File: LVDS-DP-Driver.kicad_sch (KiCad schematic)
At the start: 122 parts, among them J1 47272-0001, J2 Conn_02x15_Odd_Even, J3 Conn_01x06_Male, J4 Conn_01x03_Male, J5 Conn_01x04_Male, J6 Conn_01x03_Male, Q1 Si4816BDY, Q10 2N7002, Q2 Si4816BDY, Q3 Si4816BDY, Q4 MMBT3904, Q5 MMBT3904, Q6 2N7002, Q7 AO3401A, Q8 2N7002, Q9 2N7002, SW1 SW_DIP_x04, U1 CS5211, U2 LTC3853, U3 AT24C64

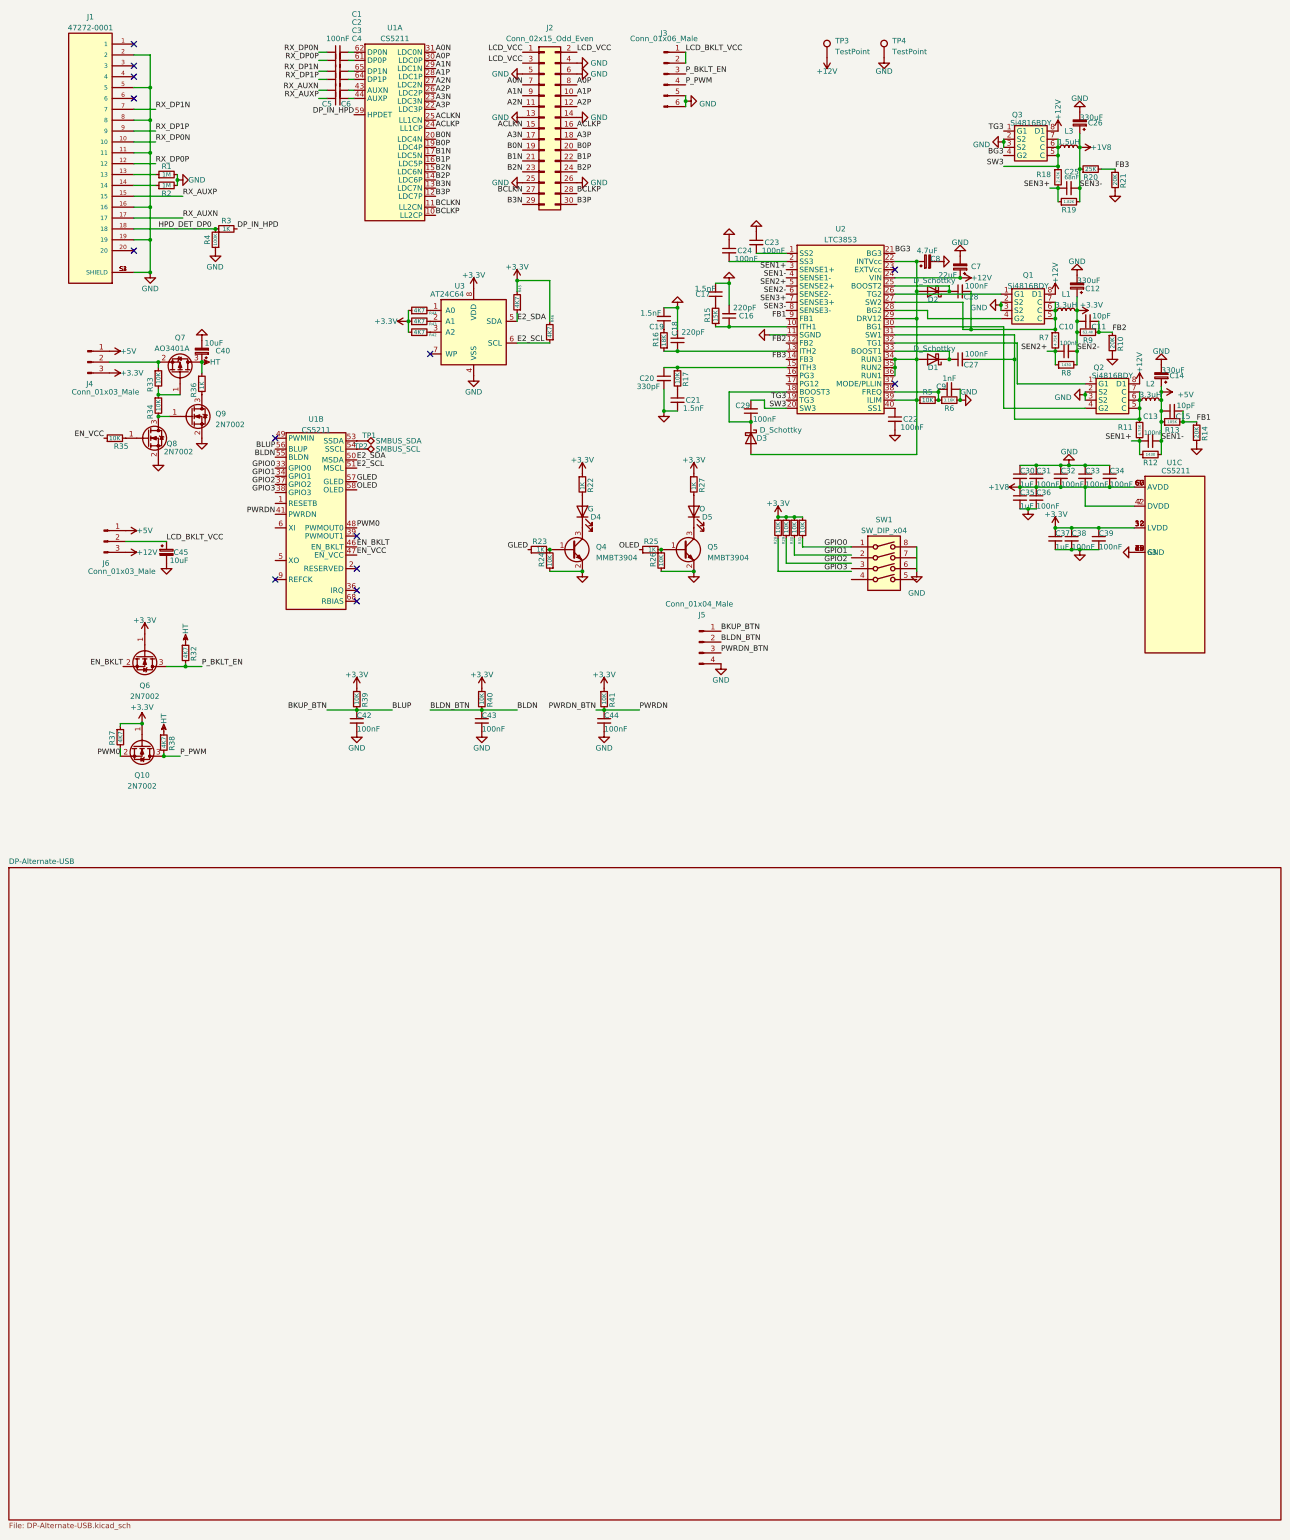
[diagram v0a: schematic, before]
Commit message: cleanup and reconstruct
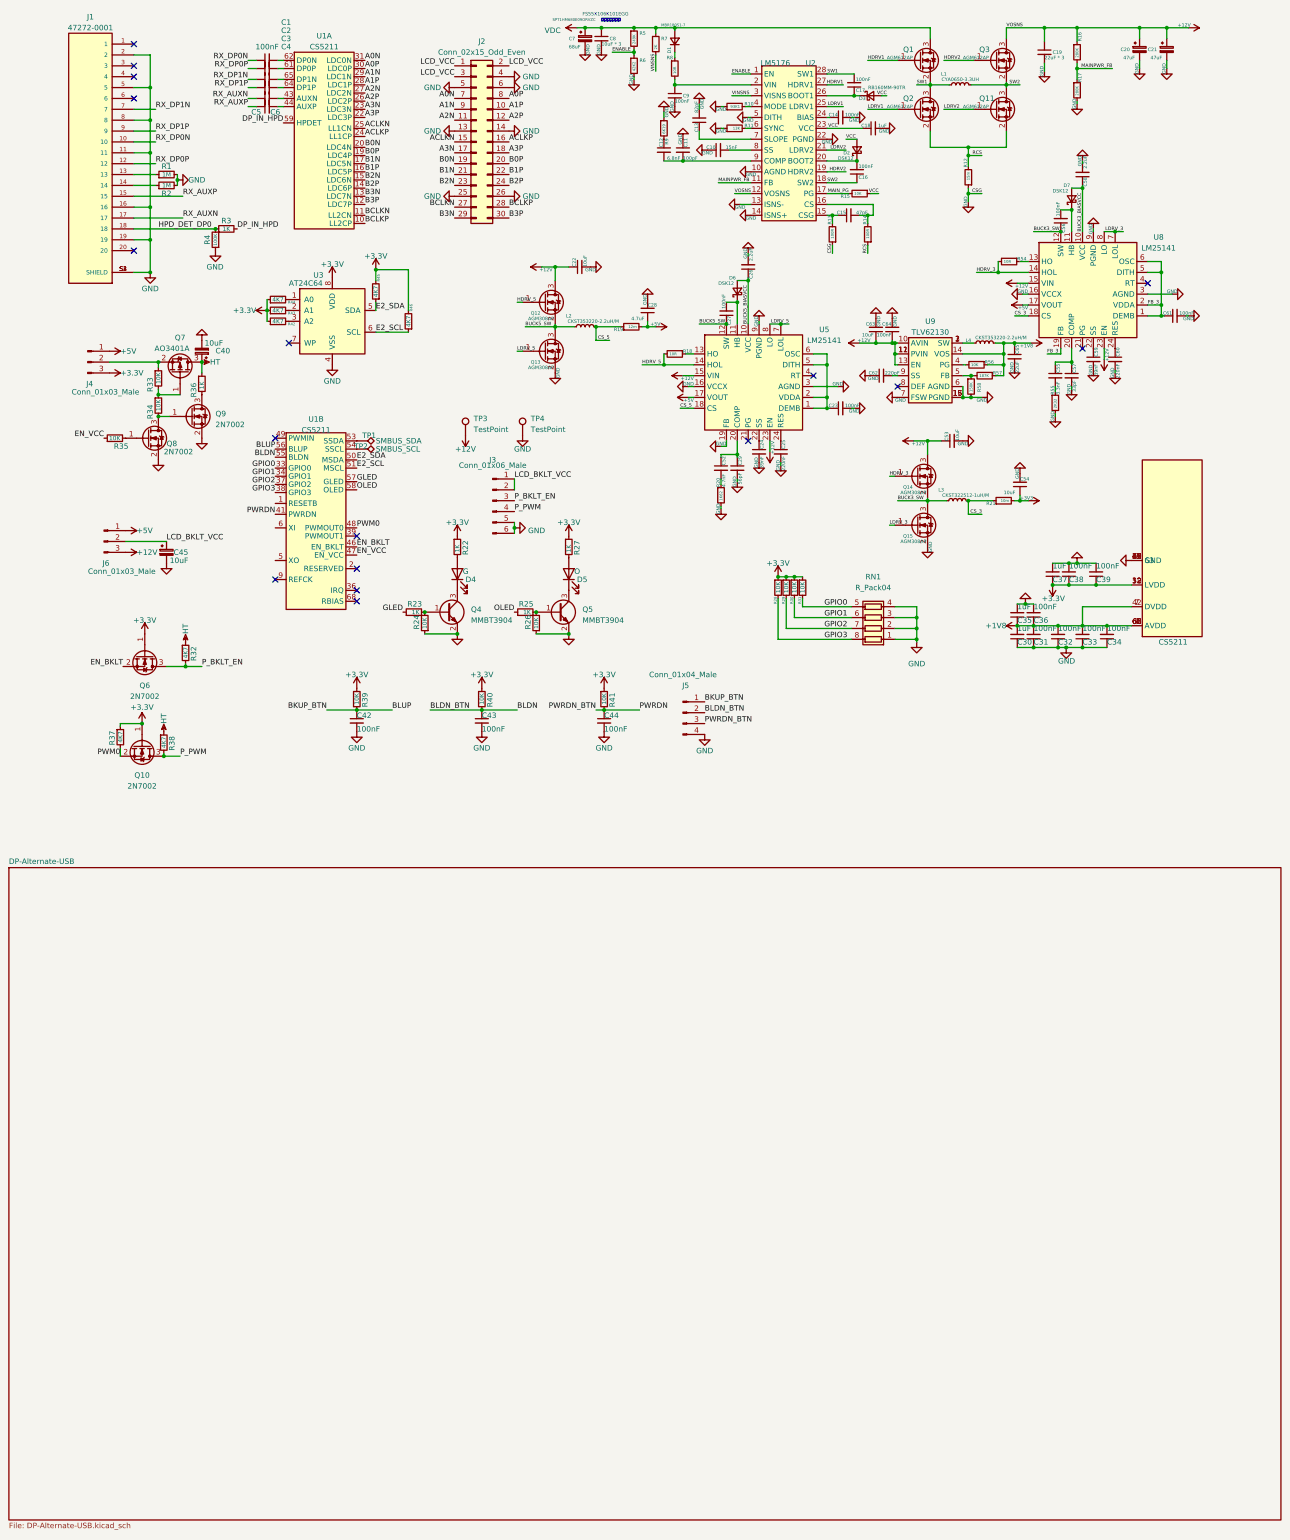
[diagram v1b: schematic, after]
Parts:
- removed C12, C14, C26: 330uF, Capacitor_Tantalum_SMD:CP_EIA-7343-31_Kemet-D, symbol Device:C_Polarized_Small
- removed C20: 330pF, Capacitor_SMD:C_0603_1608Metric, symbol Device:C_Small
- removed C21: 1.5nF, Capacitor_SMD:C_0603_1608Metric, symbol Device:C_Small
- removed C8: 4.7uF, Capacitor_Tantalum_SMD:CP_EIA-3528-21_Kemet-B, symbol Device:C_Polarized_Small
- removed D1, D2, D3: D_Schottky, Diode_SMD:D_SOD-523, symbol Device:D_Schottky
- removed Q1, Q2, Q3: Si4816BDY, Package_SO:SO-8_3.9x4.9mm_P1.27mm, symbol Symbols:Si4816BDY
- removed SW1: SW_DIP_x04, Button_Switch_THT:SW_DIP_SPSTx04_Slide_6.7x11.72mm_W7.62mm_P2.54mm_LowProfile, symbol Switch:SW_DIP_x04
- removed U2: LTC3853, Package_DFN_QFN:QFN-40-1EP_6x6mm_P0.5mm_EP4.6x4.6mm, symbol Symbols:LTC3853
- added C12: 6.8nF, Capacitor_SMD:C_0603_1608Metric, symbol Device:C_Small
- added C14, C56, C61, C64: 100nF, Capacitor_SMD:C_0603_1608Metric, symbol Device:C_Small
- added C20, C21: 47uF, Capacitor_SMD:C_1210_3225Metric, symbol Device:C_Polarized_Small
- added C26, C58: 2.2uF, Capacitor_SMD:C_0603_1608Metric, symbol Device:C_Small
- added C52: 4.7nF, Capacitor_SMD:C_0603_1608Metric, symbol Device:C_Small
- added C53, C54, C63: 10uF, Capacitor_SMD:C_0603_1608Metric, symbol Device:C_Small
- added C55: 3.3nF, Capacitor_SMD:C_0603_1608Metric, symbol Device:C_Small
- added C57: 33pF, Capacitor_SMD:C_0603_1608Metric, symbol Device:C_Small
- added C59: 39nF, Capacitor_SMD:C_0603_1608Metric, symbol Device:C_Small
- added C60: 220nF, Capacitor_SMD:C_0603_1608Metric, symbol Device:C_Small
- added C62: 220pF, Capacitor_SMD:C_0603_1608Metric, symbol Device:C_Small
- added C65: 22uF, Capacitor_SMD:C_0603_1608Metric, symbol Device:C_Small
- added C8: 10uF * 3, Capacitor_SMD:C_2220_5650Metric, symbol Device:C_Small
- added D1: MBR180S1-7, symbol Device:D_Small
- added D2, D6, D7: DSK12, Diode_SMD:D_SOD-123F, symbol Device:D_Schottky_Small
- added D3: RB160MM-90TR, Diode_SMD:D_SOD-123F, symbol Device:D_Schottky_Small
- added L4: CKST353220-2.2uH/M, symbol Device:L_Small
- added Q1, Q11, Q2, Q3: AGM612AP, symbol Device:Q_NMOS_GSD
- added Q12, Q13, Q14, Q15: AGM308AP, symbol Device:Q_NMOS_GSD
- added R54: 10R, symbol Device:R_Small
- added R55: 2K32, symbol Device:R_Small
- added R56: 10K, symbol Device:R_Small
- added R57: 187K, symbol Device:R_Small
- added R58: 150K, symbol Device:R_Small
- added RN1: R_Pack04, symbol Device:R_Pack04
- added U2: LM5176, symbol Symbols:LM5176
- added U5, U8: LM25141, symbol Symbols:LM25141
- added U9: TLV62130, symbol Symbols:TLV62130
- C10: value 100nF -> 15nF
- C11: value 10pF -> 100pF
- C13: value 100nF -> 82pF
- C15: value 10pF -> 47pF
- C16: value 220pF -> 100nF
- C17: value 1.5nF -> 100nF
- C18: value 220pF -> 1uF
- C19: value 1.5nF -> 22uF * 3; footprint Capacitor_SMD:C_0603_1608Metric -> Capacitor_SMD:C_0805_2012Metric
- C22: value 100nF -> 10uF
- C24: value 100nF -> 39nF
- C25: value 68nF -> 220nF
- C28: value 100nF -> 4.7uF
- C29: value 100nF -> 56pF
- C7: value 22uF -> 68uF; footprint Capacitor_Tantalum_SMD:CP_EIA-3528-21_Kemet-B -> Capacitor_THT:CP_Radial_D6.3mm_P2.50mm
- C9: value 1nF -> 100nF
- J1: footprint MOLEX_47272-0001 -> Footprints:MOLEX_47272-0001
- L1: value 3.3uH -> CYA0650-3.3UH; footprint Inductor_SMD:L_7.3x7.3_H4.5 -> (none)
- L2: value 3.3uH -> CKST353220-2.2uH/M; footprint Inductor_SMD:L_7.3x7.3_H4.5 -> (none)
- L3: value 1.5uH -> CKST322512-1uH/M; footprint Inductor_SMD:L_1210_3225Metric -> (none)
- R10: value 20K -> 93K1; footprint Resistor_SMD:R_0603_1608Metric -> (none)
- R11: value 4.75K -> 13K; footprint Resistor_SMD:R_0603_1608Metric -> (none)
- R12: value 1430 -> 15m; footprint Resistor_SMD:R_1206_3216Metric -> (none)
- R13: value 105K -> 100R; footprint Resistor_SMD:R_0603_1608Metric -> (none)
- R14: value 20K -> 100R; footprint Resistor_SMD:R_0603_1608Metric -> (none)
- R15: value 15K -> 10K; footprint Resistor_SMD:R_0603_1608Metric -> (none)
- R16: value 18K -> 280K; footprint Resistor_SMD:R_0603_1608Metric -> (none)
- R17: value 10K -> 280K; footprint Resistor_SMD:R_0603_1608Metric -> (none)
- R18: value 2.43K -> 10R; footprint Resistor_SMD:R_0603_1608Metric -> (none)
- R19: value 1.82K -> 12m; footprint Resistor_SMD:R_0603_1608Metric -> (none)
- R20: value 25K -> 1K62; footprint Resistor_SMD:R_0603_1608Metric -> (none)
- R21: value 20K -> 10m; footprint Resistor_SMD:R_0603_1608Metric -> (none)
- R5: value 10K -> 249K; footprint Resistor_SMD:R_0603_1608Metric -> (none)
- R6: value 3.16K -> 42K2; footprint Resistor_SMD:R_0603_1608Metric -> (none)
- R7: value 4.75K -> 2K; footprint Resistor_SMD:R_0603_1608Metric -> (none)
- R8: value 1430 -> 10R; footprint Resistor_SMD:R_1206_3216Metric -> (none)
- R9: value 63.4K -> 6K19; footprint Resistor_SMD:R_0603_1608Metric -> (none)
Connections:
- net +12V: now also C19.1, C22.1, R16.1, C20.1, C21.1, C53.1, C63.1, C64.1, Q12.3 (D), Q14.3 (D), Q3.3 (D), U2.12 (VOSNS), U5.15 (VIN), U5.23 (EN), U8.15 (VIN), U8.23 (EN), U9.10 (AVIN), U9.11 (PVIN), U9.12 (PVIN), U9.13 (EN); no longer C7.1
- net +1V8: now also C65.1, L4.2, R56.1, R57.1, U9.14 (VOS); no longer C25.2, L3.2, R19.2, R20.1
- net +3.3V: no longer C10.2, C11.1, L1.2, R8.2, R9.1
- net +5V: now also C28.1, R19.2, U5.17 (VOUT), U8.17 (VOUT); no longer C13.2, C15.1, L2.2, R12.2, R13.1
- net GND: now also C10.1, C11.1, C13.2, C23.2, C24.2, C25.2, C28.2, C29.2, R10.1, R11.1, R12.1, R13.1, R17.2, R20.2, R9.1, C14.2, C20.2, C21.2, C26.2, C53.2, C54.2, C57.2, C58.2, C59.2, C60.2, C61.2, C62.1, C63.2, C64.2, C65.2, C8.2, Q13.2 (S), Q15.2 (S), R55.2, R58.2, RN1.1 (R1.1), RN1.2 (R2.1), RN1.3 (R3.1), RN1.4 (R4.1), U2.10 (AGND), U2.13 (ISNS-), U2.14 (ISNS+), U2.22 (PGND), U2.5 (DITH), U5.16 (VCCX), U5.19 (FB), U5.3 (AGND), U5.9 (PGND), U8.16 (VCCX), U8.3 (AGND), U8.9 (PGND), U9.15 (PGND), U9.16 (PGND), U9.17 (PGND), U9.6 (AGND), U9.7 (FSW); no longer C16.2, C17.2, C23.1, C24.1, R10.2, R14.2, R21.2
- net GPIO0: now also RN1.5 (R4.2)
- net GPIO1: now also RN1.6 (R3.2)
- net GPIO2: now also RN1.7 (R2.2)
- net GPIO3: now also RN1.8 (R1.2)
- net ENABLE: now reaches R5.2, R6.1
- net ENABLE: now also U2.1 (EN); no longer C9.1
- net MAINPWR_FB: now reaches R17.1
- net MAINPWR_FB: now also R16.2, U2.11 (FB)
- net BUCK5_SW: now reaches C27.1
- net BUCK5_SW: now also L2.1, Q12.2 (S), Q13.3 (D), U5.12 (SW)
- net VDC: now reaches R5.1
- net VDC: now also C7.1, R7.1, C8.1, D1.2 (A), Q1.3 (D)
- net VCC: now reaches C18.1
- net VCC: now also R15.1, D2.2 (A), D3.2 (A), U2.23 (VCC); no longer R16.1
- net at C29.1: now also C52.1, U5.20 (COMP)
- net at C17.1: now also D3.1 (K), U2.26 (BOOT1); no longer R15.2
- net SW2: now reaches C16.1
- net SW2: now also L1.2, Q11.3 (D), Q3.2 (S), U2.18 (SW2); no longer R15.1
- removed net FB1: C15.2, R13.2, R14.1
- removed net FB2: C11.2, R10.1, R9.2
- net FB3 renamed CS_3
- net CS_3: now also L3.2, U8.18 (CS); no longer R20.2
- removed net SEN1+: C13.1, R11.2, R12.1
- removed net SEN2+: C10.1, R7.2, R8.1
- removed net SEN3+: C25.1, R18.2, R19.1
- removed net SW3: C29.2, L3.1, R18.1
- new net: C13.1, U2.7 (SLOPE)
- new net: C12.1, R9.2
- new net: C10.2, U2.8 (SS)
- new net: R54.1, U8.13 (HO)
- new net: C25.1, U5.24 (RES)
- new net: C56.2, D7.1 (K), U8.11 (HB)
- new net: R56.2, U9.4 (PG)
- new net: C62.2, U9.9 (SS)
- new net: C27.2, D6.1 (K), U5.11 (HB)
- new net: C52.2, R20.1
- new net: C11.2, C12.2, U2.9 (COMP)
- new net: R11.2, U2.6 (SYNC)
- new net: C59.1, U8.22 (SS)
- new net: C15.2, R14.2, U2.16 (CS)
- new net: R57.2, R58.1, U9.5 (FB)
- new net: R18.1, U5.13 (HO)
- new net: C60.1, U8.24 (RES)
- new net: C9.1, R8.2, U2.2 (VIN)
- new net: C23.1, U5.1 (DEMB), U5.2 (VDDA), U5.5 (DITH), U5.6 (OSC)
- new net: C24.1, U5.22 (SS)
- new net: L4.1, U9.1 (SW), U9.2 (SW), U9.3 (SW)
- new net: R10.2, U2.4 (MODE)
- new net: C55.1, C57.1, U8.20 (COMP)
- new net: C16.2, D2.1 (K), U2.20 (BOOT2)
- new net: D1.1 (K), R8.1
- new net: C55.2, R55.1
- new net: C15.1, R13.2, U2.15 (CSG)
- new net: C14.1, U2.24 (BIAS)
- new net +3V3: C54.1, R21.2
- new net BUCK3_BIASVCC: C58.1, D7.2 (A), U8.10 (VCC)
- new net BUCK3_SW: C56.1, L3.1, Q14.2 (S), Q15.3 (D), U8.12 (SW)
- new net BUCK5_BIASVCC: C26.1, D6.2 (A), U5.10 (VCC)
- new net CS_5: L2.2, R19.1, U5.18 (CS)
- new net FB_3: C61.1, U8.1 (DEMB), U8.19 (FB), U8.2 (VDDA), U8.5 (DITH), U8.6 (OSC)
- new net HDRV1: Q1.1 (G), U2.27 (HDRV1)
- new net HDRV2: Q3.1 (G), U2.19 (HDRV2)
- new net HDRV_3: Q14.1 (G), R54.2, U8.14 (HOL)
- new net HDRV_5: Q12.1 (G), R18.2, U5.14 (HOL)
- new net LDRV1: Q2.1 (G), U2.25 (LDRV1)
- new net LDRV2: Q11.1 (G), U2.21 (LDRV2)
- new net LDRV_3: Q15.1 (G), U8.7 (LOL), U8.8 (LO)
- new net LDRV_5: Q13.1 (G), U5.7 (LOL), U5.8 (LO)
- new net MAIN_PG: R15.2, U2.17 (PG)
- new net RCS: Q11.2 (S), Q2.2 (S), R12.2, R14.1
- new net SW1: C17.2, L1.1, Q1.2 (S), Q2.3 (D), U2.28 (SW1)
- new net VINSNS: R7.2, U2.3 (VISNS)
- no-connect marks 14 -> 17
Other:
- note added: "FS55X106K101EGG"
- note added: "SPT1HM680E09ORVZC"
- note added: "同焊盘堆叠焊接"
- moved on the sheet: C1, C2, C3, C30, C31, C32, C33, C34, C35, C36, C37, C38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
